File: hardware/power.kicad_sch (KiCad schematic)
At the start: 18 parts, among them U2 AOZ1280CI, U3 LM1117-5.0, U4 LM1117-3.3

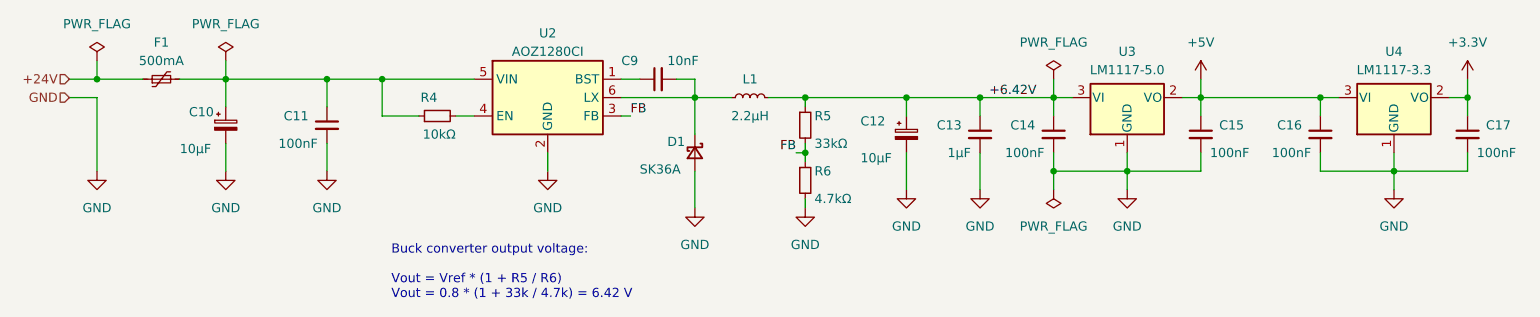
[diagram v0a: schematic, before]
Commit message: Apply KiCad template to the project
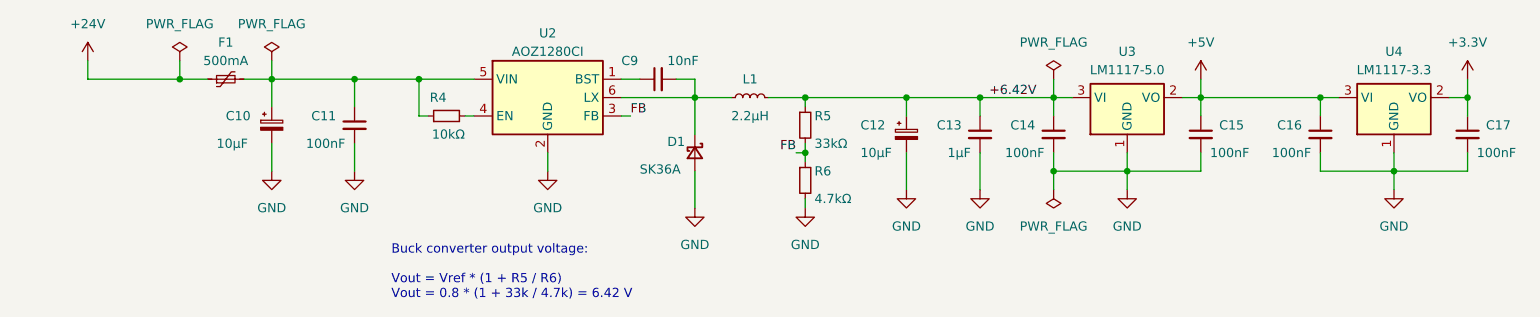
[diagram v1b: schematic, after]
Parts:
- U3: symbol Regulator_Linear:LM1117-5.0 -> Regulator_Linear:LM1117MP-5.0
- U4: symbol Regulator_Linear:LM1117-3.3 -> Regulator_Linear:LM1117MP-3.3
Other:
- moved on the sheet: C10, C11, F1, R4
